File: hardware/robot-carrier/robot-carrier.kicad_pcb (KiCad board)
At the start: 2 copper layers, 60 x 73.5 mm, 36 parts, among them J1 DB128L BAT IN, LCSC C500021, J10 M1, J11 M2, J12 M3, J13 M4, J2 DB128L 2P, LCSC C500021, J20 S1, J21 S2, J22 S3, J23 S4, J3 DB128L 2P, LCSC C500021, J30 IMU I2C, J40 GA25-370 L298N: ENA / IN1 / I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, J41 DB128L 3P, LCSC C430602

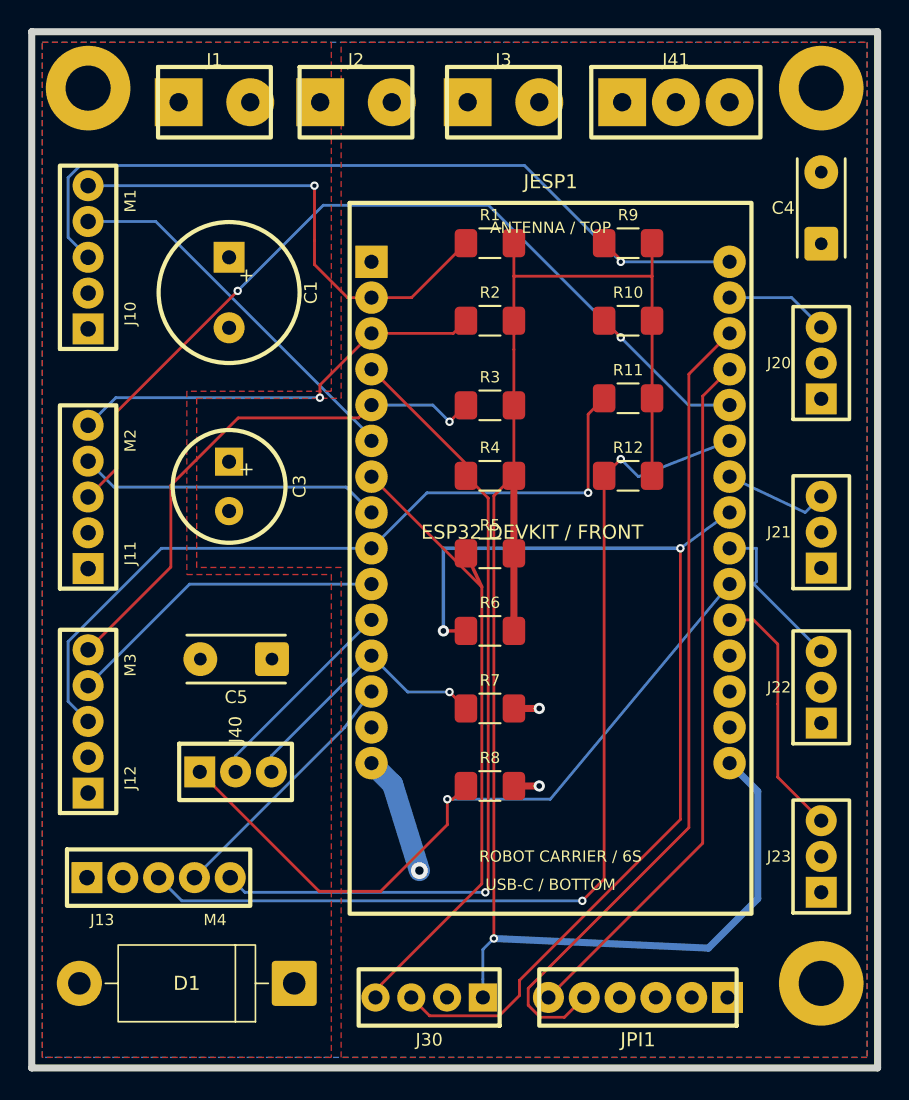
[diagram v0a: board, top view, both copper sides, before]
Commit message: updated
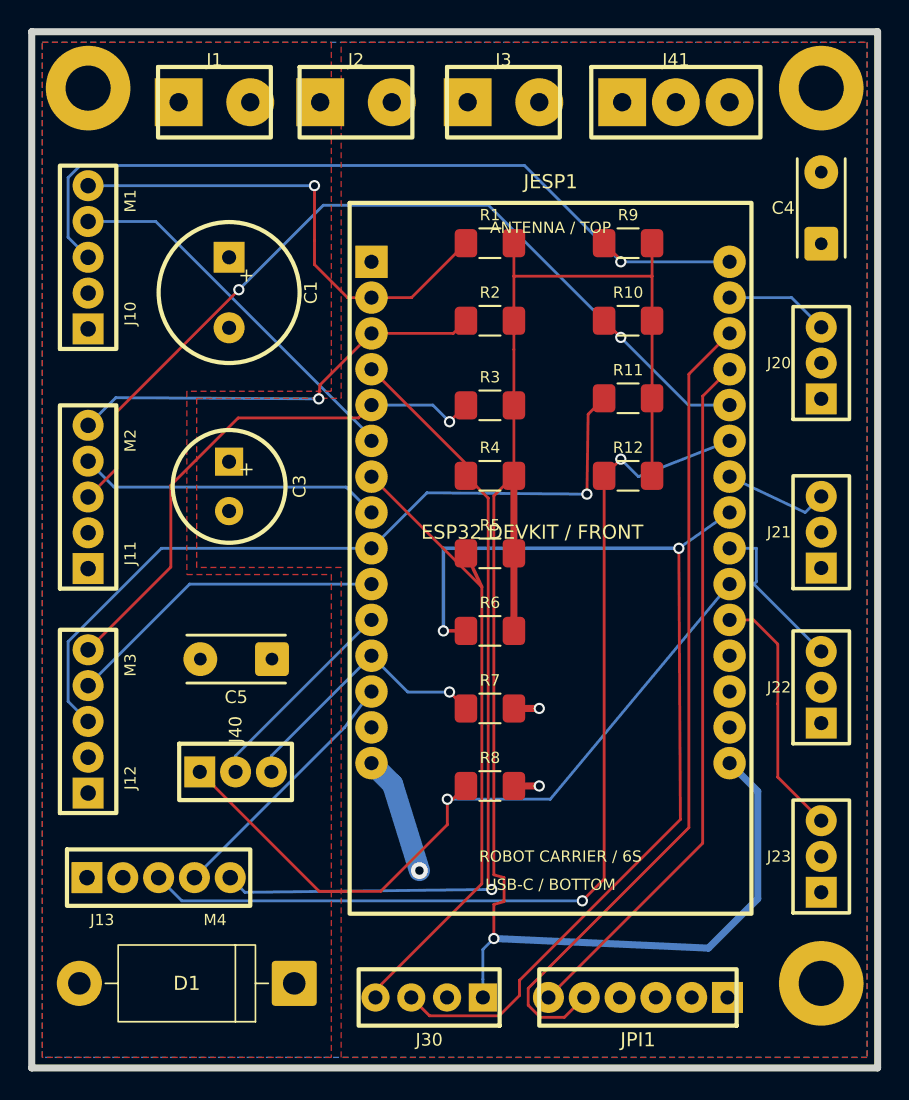
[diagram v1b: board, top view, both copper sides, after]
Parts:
- C3: value 1000uF 10V, LCSC C79119 -> 1000uF 16V, LCSC C51934166
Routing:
- net +3V3: track 122.3 -> 123.4 mm
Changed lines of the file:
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@@
 			)
 		)
-		(property "Value" "1000uF 10V, LCSC C79119"
+		(property "Value" "1000uF 16V, LCSC C51934166"
 			(at 0 5 90)
 			(layer "F.Fab")
@@
 			)
 		)
-		(property "LCSC" "C79119"
+		(property "LCSC" "C51934166"
 			(at 0 0 90)
 			(layer "F.Fab")
@@
 		(at 56 68)
 		(size 0.8)
-		(drill 0.4)
+		(drill 0.5)
 		(layers "F.Cu" "B.Cu")
 		(net "GND")
@@
 		(at 56 73.5)
 		(size 0.8)
-		(drill 0.4)
+		(drill 0.5)
 		(layers "F.Cu" "B.Cu")
 		(net "GND")
@@
 	(segment
 		(start 59.4669 47.1331)
-		(end 59.4669 52.7035)
+		(end 59.38 52.8)
 		(width 0.2)
 		(layer "F.Cu")
@@
 	)
 	(via
-		(at 59.4669 52.7035)
-		(size 0.6)
-		(drill 0.3)
+		(at 59.38 52.8)
+		(size 0.8)
+		(drill 0.5)
 		(layers "F.Cu" "B.Cu")
 		(net "M3_PWM_3V3")
 	)
 	(segment
-		(start 59.4669 52.7035)
+		(start 59.38 52.8)
 		(end 48.0365 52.7035)
 		(width 0.2)
@@
 	(segment
 		(start 52.7793 84.3173)
-		(end 52.7793 52.9207)
+		(end 52.7793 81.9)
 		(width 0.2)
 		(layer "F.Cu")
@@
 	)
 	(segment
+		(start 53.5 81.7)
+		(end 53.5 80)
+		(width 0.2)
+		(layer "F.Cu")
+		(net "+3V3")
+	)
+	(segment
 		(start 64 37.3428)
 		(end 64 35)
@@
 		(start 54.2 46.5)
 		(end 54.2 51.5)
+		(width 0.2)
+		(layer "F.Cu")
+		(net "+3V3")
+	)
+	(segment
+		(start 52.7793 79.8)
+		(end 52.7793 52.9207)
 		(width 0.2)
 		(layer "F.Cu")
@@
 		(net "+3V3")
 	)
+	(segment
+		(start 53.5 80)
+		(end 52.7793 79.8)
+		(width 0.2)
+		(layer "F.Cu")
+		(net "+3V3")
+	)
+	(segment
+		(start 52.7793 81.9)
+		(end 53.5 81.7)
+		(width 0.2)
+		(layer "F.Cu")
+		(net "+3V3")
+	)
 	(via
 		(at 52.7793 84.3173)
-		(size 0.6)
-		(drill 0.3)
+		(size 0.8)
+		(drill 0.5)
 		(layers "F.Cu" "B.Cu")
 		(net "+3V3")
@@
 	(via
 		(at 40.0545 30.92)
-		(size 0.6)
-		(drill 0.3)
+		(size 0.8)
+		(drill 0.5)
 		(layers "F.Cu" "B.Cu")
 		(net "M1_ENC")
@@
 	(segment
 		(start 66.0101 75.8725)
-		(end 66.0101 56.64)
+		(end 65.9 56.64)
 		(width 0.2)
 		(layer "F.Cu")
@@
 	)
 	(via
-		(at 66.0101 56.64)
-		(size 0.6)
-		(drill 0.3)
+		(at 65.9 56.64)
+		(size 0.8)
+		(drill 0.5)
 		(layers "F.Cu" "B.Cu")
 		(net "IMU_I2C_SCL_3V3")
@@
 		(at 49.2 62.5)
 		(size 0.8)
-		(drill 0.4)
+		(drill 0.5)
 		(layers "F.Cu" "B.Cu")
 		(net "IMU_I2C_SCL_3V3")
@@
 	(segment
 		(start 69.5 54.1)
-		(end 66.0101 56.64)
+		(end 65.9 56.64)
 		(width 0.2)
 		(layer "B.Cu")
@@
 	(via
 		(at 59.0548 81.6448)
-		(size 0.6)
-		(drill 0.3)
+		(size 0.8)
+		(drill 0.5)
 		(layers "F.Cu" "B.Cu")
 		(net "M4_PWM_3V3")
@@
 	(via
 		(at 61.7828 50.3172)
-		(size 0.6)
-		(drill 0.3)
+		(size 0.8)
+		(drill 0.5)
 		(layers "F.Cu" "B.Cu")
 		(net "M4_PWM_3V3")
@@
 	(segment
 		(start 52.3775 80.8404)
-		(end 52.1754 81.0425)
+		(end 52.63 80.84)
 		(width 0.2)
 		(layer "F.Cu")
@@
 	)
 	(via
-		(at 52.1754 81.0425)
-		(size 0.6)
-		(drill 0.3)
+		(at 52.63 80.84)
+		(size 0.8)
+		(drill 0.5)
 		(layers "F.Cu" "B.Cu")
 		(net "M4_ENC")
@@
 	(segment
 		(start 35.1225 81.0425)
-		(end 52.1754 81.0425)
+		(end 52.63 80.84)
 		(width 0.2)
 		(layer "B.Cu")
@@
 	(via
 		(at 61.7817 36.32)
-		(size 0.6)
-		(drill 0.3)
+		(size 0.8)
+		(drill 0.5)
 		(layers "F.Cu" "B.Cu")
 		(net "M1_PWM_3V3")
@@
 	(segment
 		(start 40.4403 45.0597)
-		(end 40.4403 45.9586)
+		(end 40.36 46.04)
 		(width 0.2)
 		(layer "F.Cu")
@@
 	)
 	(via
-		(at 40.4403 45.9586)
-		(size 0.6)
-		(drill 0.3)
+		(at 40.36 46.04)
+		(size 0.8)
+		(drill 0.5)
 		(layers "F.Cu" "B.Cu")
 		(net "M2_ENC")
@@
 	)
 	(segment
-		(start 40.4403 45.9586)
+		(start 40.36 46.04)
 		(end 25.9614 45.9586)
 		(width 0.2)
@@
 	(via
 		(at 49.6357 47.6643)
-		(size 0.6)
-		(drill 0.3)
+		(size 0.8)
+		(drill 0.5)
 		(layers "F.Cu" "B.Cu")
 		(net "M3_ENC")
@@
 	(via
 		(at 49.6346 66.8346)
-		(size 0.6)
-		(drill 0.3)
+		(size 0.8)
+		(drill 0.5)
 		(layers "F.Cu" "B.Cu")
 		(net "GA25_IN2_3V3")
@@
 	)
 	(segment
-		(start 34.6088 38.3821)
+		(start 34.69 38.3)
 		(end 26.0472 46.9437)
 		(width 0.2)
@@
 	(via
 		(at 61.7809 41.6809)
-		(size 0.6)
-		(drill 0.3)
+		(size 0.8)
+		(drill 0.5)
 		(layers "F.Cu" "B.Cu")
 		(net "M2_PWM_3V3")
 	)
 	(via
-		(at 34.6088 38.3821)
-		(size 0.6)
-		(drill 0.3)
+		(at 34.69 38.3)
+		(size 0.8)
+		(drill 0.5)
 		(layers "F.Cu" "B.Cu")
 		(net "M2_PWM_3V3")
@@
 	)
 	(segment
-		(start 34.6088 38.3821)
+		(start 34.69 38.3)
 		(end 40.6832 32.3077)
 		(width 0.2)
@@
 	(via
 		(at 49.4783 74.438)
-		(size 0.6)
-		(drill 0.3)
+		(size 0.8)
+		(drill 0.5)
 		(layers "F.Cu" "B.Cu")
 		(net "GA25_ENA_PWM_3V3")
